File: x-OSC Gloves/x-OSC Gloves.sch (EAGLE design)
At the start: 32 parts

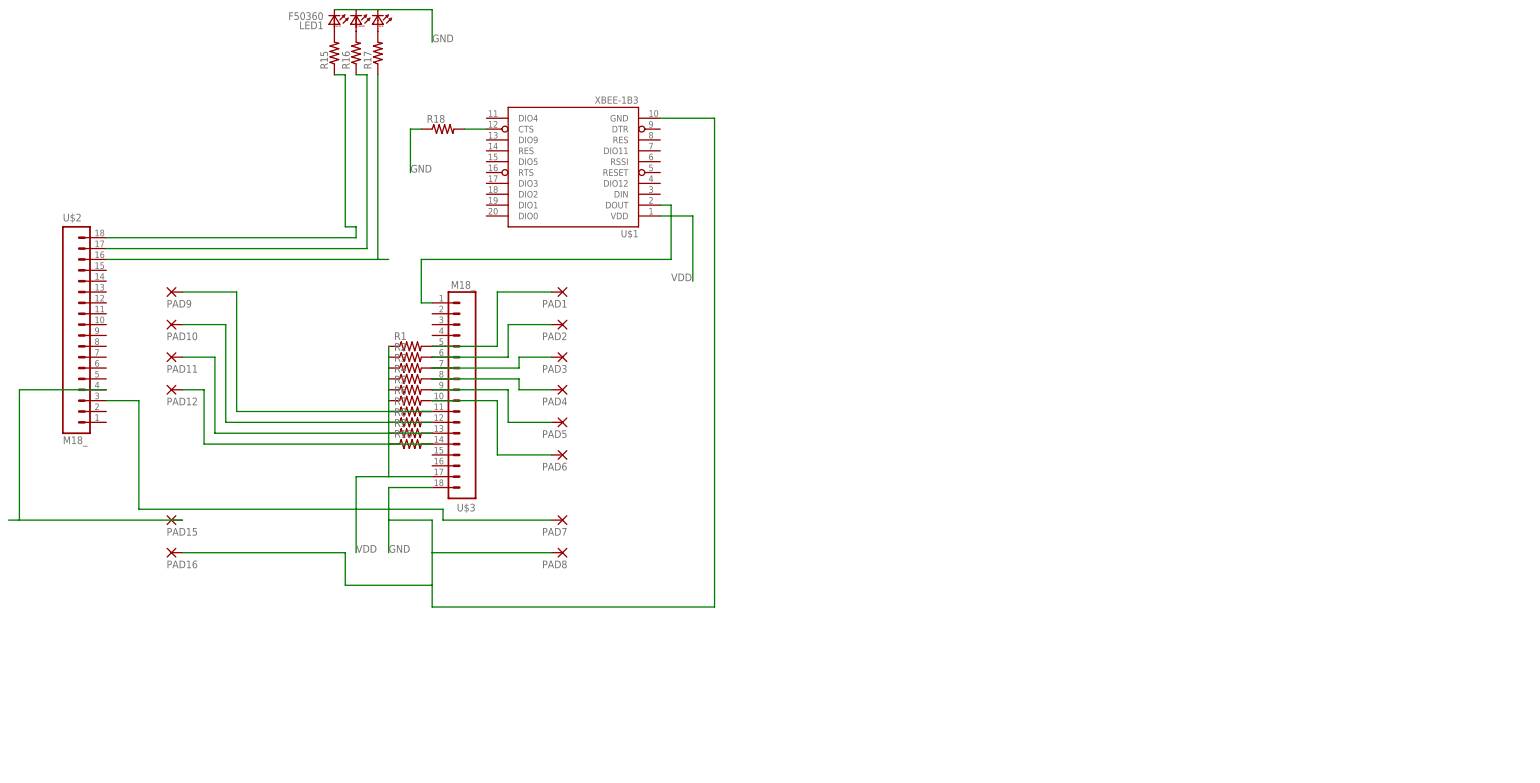
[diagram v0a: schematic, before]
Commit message: xOSC circuit
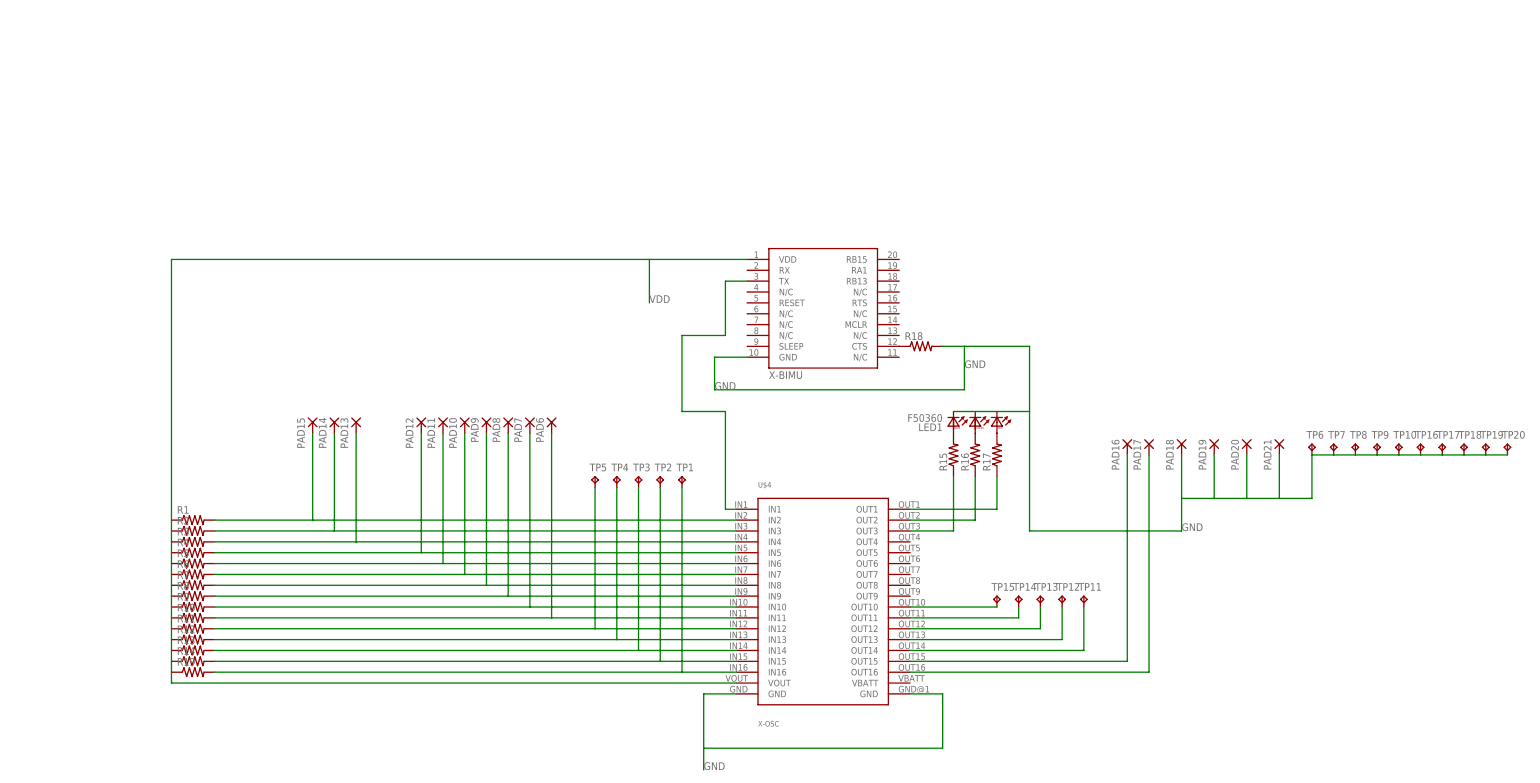
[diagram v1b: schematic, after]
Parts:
- removed PAD1, PAD2, PAD3, PAD4, PAD5: (no value), wirepad:3,81/1,4
- removed U$1: XBEE-1B3, SparkFun-RF:XBEE-1B3
- removed U$2, U$3: M18_, SparkFun-Connectors:M18_
- added PAD13, PAD14, PAD17, PAD18, PAD19, PAD20, PAD21: (no value), wirepad:3,81/1,4
- added R11, R12, R13, R14, R19: (no value), SparkFun-Passives:RESISTOR0805-RES
- added TP1, TP10, TP11, TP12, TP13, TP14, TP15, TP16, TP17, TP18, TP19, TP2, TP20, TP3, TP4, TP5, TP6, TP7, TP8, TP9: TPTP20R, testpad:TPTP20R
- added U$4: X-OSC, x-io:X-OSC
- added U$5: X-BIMU, x-io:X-BIMU
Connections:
- new net N$10: R18.1, U$5.CTS
- new net N$11: U$4.IN1, U$5.TX
- new net N$23: PAD16.P, U$4.OUT15
- new net N$24: PAD17.P, U$4.OUT16
- new net N$25: R17.1, U$4.OUT1
- new net N$26: TP11.TP, U$4.OUT14
- new net N$29: TP12.TP, U$4.OUT13
- new net N$30: TP13.TP, U$4.OUT12
- new net N$31: TP14.TP, U$4.OUT11
- new net N$32: TP15.TP, U$4.OUT10
- net GND: now also PAD18.P, PAD19.P, PAD20.P, PAD21.P, R18.2, TP10.TP, TP16.TP, TP17.TP, TP18.TP, TP19.TP, TP20.TP, TP6.TP, TP7.TP, TP8.TP, TP9.TP, U$4.GND, U$4.GND@1, U$5.GND; no longer PAD16.P, PAD8.P, R18.1, U$1.GND, U$3.18
- net N$12: now also PAD10.P, R6.2, U$4.IN7; no longer R17.1, U$2.16
- net N$13: now also PAD9.P, R7.2, U$4.IN8; no longer PAD2.P, R2.2, U$3.6
- net N$14: now also PAD8.P, R8.2, U$4.IN9; no longer R18.2, U$1.CTS
- net N$15: now also R9.2, U$4.IN10; no longer U$2.3
- net N$16: now also PAD6.P, R10.2, U$4.IN11; no longer PAD15.P, U$2.4
- net N$18: now also R11.2, TP5.TP, U$4.IN12; no longer R15.1, U$2.18
- net N$19: now also R12.2, TP4.TP, U$4.IN13; no longer R16.1, U$2.17
- net N$20: now also R13.2, TP3.TP, U$4.IN14; no longer PAD12.P, R10.2, U$3.14
- net N$21: now also R14.2, TP2.TP, U$4.IN15; no longer PAD1.P, R1.2, U$3.5
- net N$22: now also R19.2, TP1.TP, U$4.IN16; no longer U$1.DOUT, U$3.1
- net N$3: now also R15.1, U$4.OUT3; no longer PAD3.P, R3.2, U$3.7
- net N$4: now also PAD15.P, R1.2, U$4.IN2; no longer PAD4.P, R4.2, U$3.8
- net N$5: now also R16.1, U$4.OUT2; no longer PAD5.P, R5.2, U$3.9
- net N$6: now also PAD14.P, R2.2, U$4.IN3; no longer PAD6.P, R6.2, U$3.10
- net N$7: now also PAD13.P, R3.2, U$4.IN4; no longer PAD9.P, R7.2, U$3.11
- net N$8: now also PAD12.P, R4.2, U$4.IN5; no longer PAD10.P, R8.2, U$3.12
- net N$9: now also R5.2, U$4.IN6; no longer R9.2, U$3.13
- net VDD: now also R11.1, R12.1, R13.1, R14.1, R19.1, U$4.VOUT, U$5.VDD; no longer U$1.VDD, U$3.17
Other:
- moved on the sheet: LED1, PAD10, PAD11, PAD12, PAD15, PAD16, PAD6, PAD7, PAD8, PAD9, R1, R10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
